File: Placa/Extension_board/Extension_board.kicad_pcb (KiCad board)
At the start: 2 copper layers, 40.6 x 24.1 mm, 8 parts, among them J1 USB_B_Micro, J2 USB_B_Micro, J3 Conn_01x06_Male, U1 STEVAL-STLCS01V1

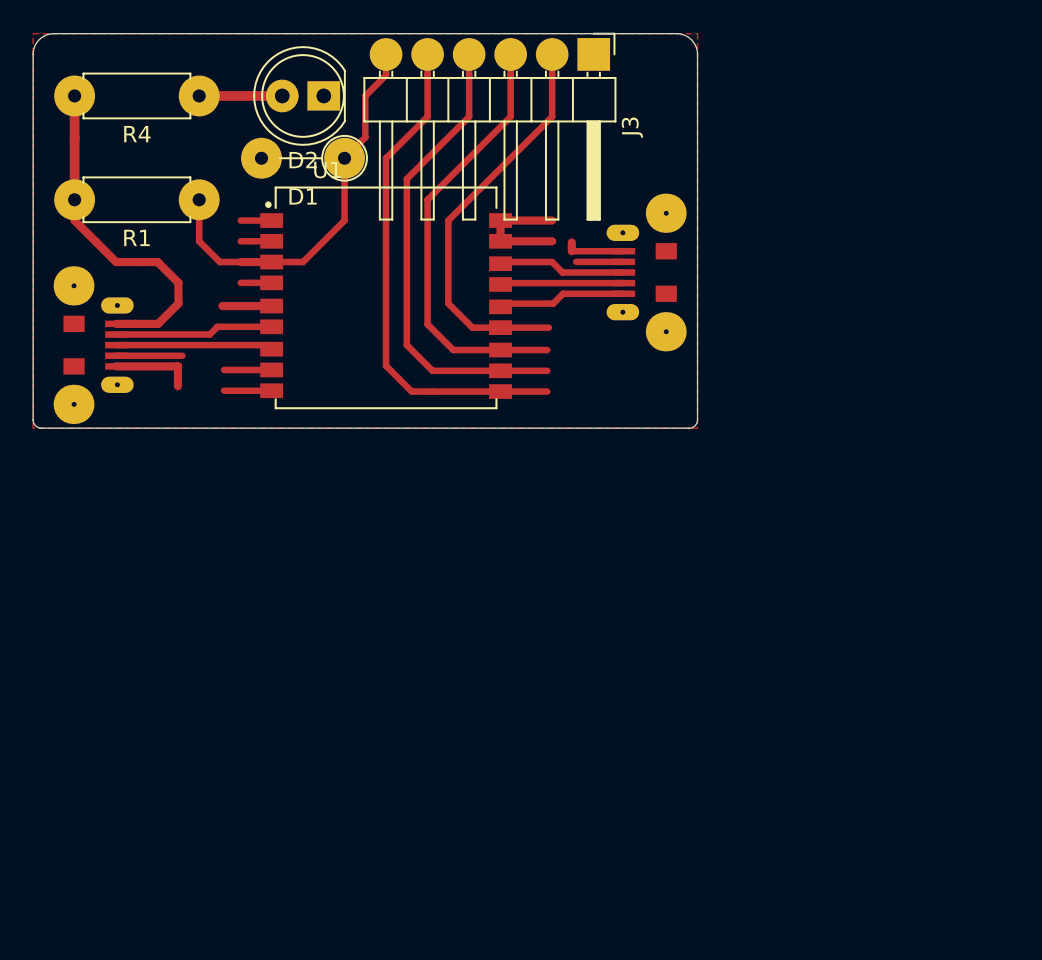
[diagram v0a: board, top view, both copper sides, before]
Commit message: Revision
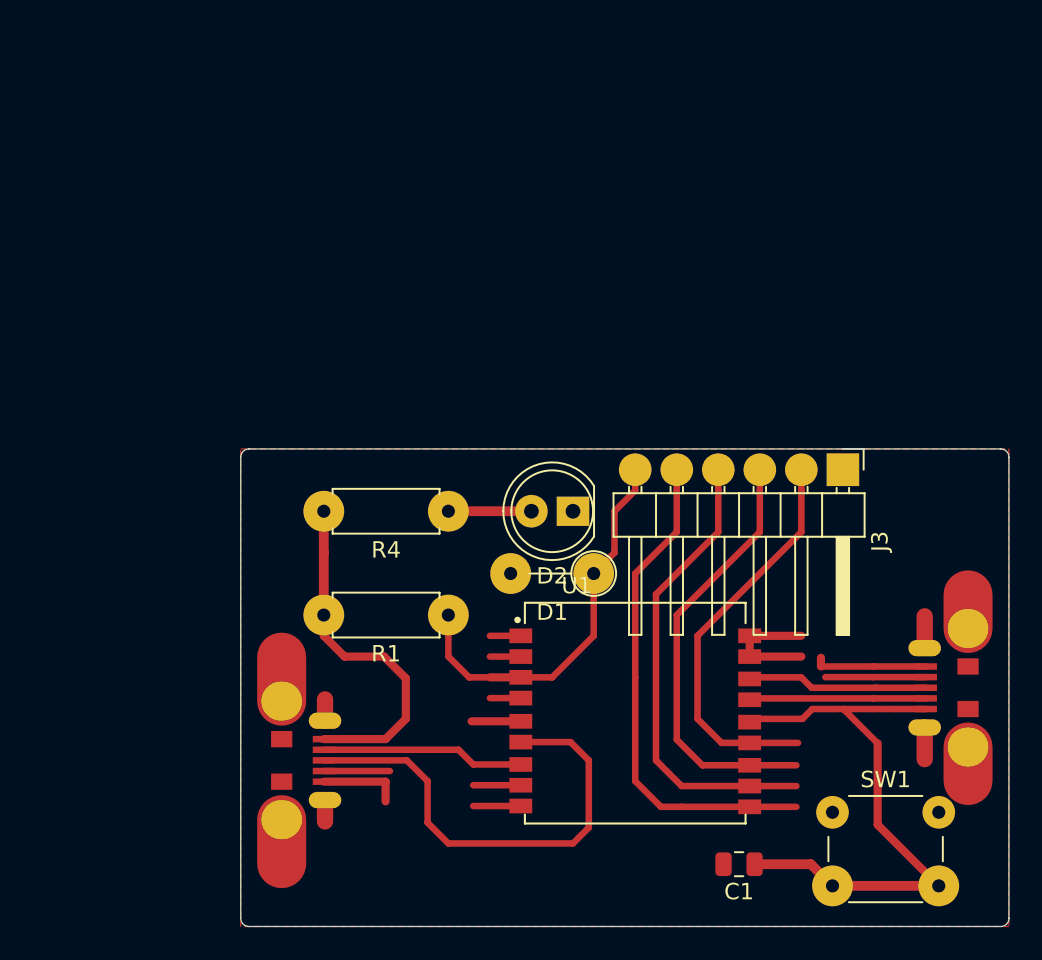
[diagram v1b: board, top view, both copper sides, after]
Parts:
- added C1: C, Capacitor_SMD:C_0805_2012Metric, F.Cu at (141.0, 86.4)
- added SW1: SW_PUSHBUTTON, Button_Switch_THT:SW_PUSH_6mm_H5mm, F.Cu at (146.7, 83.2)
- moved J1 31.4 mm to (152.4, 75.6)
- moved D1 29.6 mm to (132.1, 68.6)
- moved D2 29.6 mm to (130.8, 64.8)
- moved U1 29.6 mm to (134.6, 77.5)
- moved R1 29.6 mm to (123.2, 71.1)
- moved R4 29.6 mm to (123.2, 64.8)
- moved J3 29.6 mm to (147.3, 62.2)
- moved J2 28.4 mm to (115.6, 80.0)
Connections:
- J2 pad 2: /RXD-USB_DP -> /RXD-USB_DM
- J2 pad 3: /RXD-USB_DM -> /RXD-USB_DP
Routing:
- net /RESET: track 7.89 -> 36.2 mm
- net /RXD-USB_DP: track 9.70 -> 28.9 mm
- net (no net): track 0.00 -> 16.9 mm
- net /GND: track 19.3 -> 22.5 mm
- net /SWDCLK: track 7.57 -> 10.8 mm
- net Net-(J1-Pad4): track 2.93 -> 6.15 mm
- net /SWDIO: track 7.87 -> 11.1 mm
- net /RXD-USB_DM: track 9.61 -> 12.8 mm
- net /V_USB: track 21.1 -> 21.7 mm
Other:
- board size 40.6 x 24.1 mm -> 47 x 29.2 mm
